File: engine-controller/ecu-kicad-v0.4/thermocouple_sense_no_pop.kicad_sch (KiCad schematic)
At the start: 5 parts, among them U1 AD8495

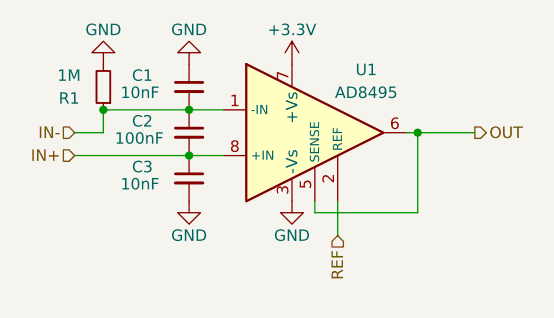
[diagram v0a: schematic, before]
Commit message: Progress on ECU v0.4
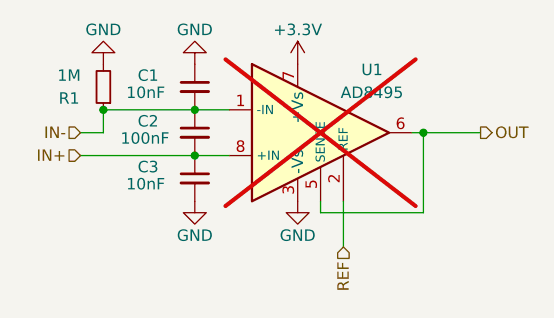
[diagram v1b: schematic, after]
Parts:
- U1: footprint Package_SO:MSOP-8_3x3mm_P0.65mm -> CustomFootprints:MSOP-8_3x3mm_P0.65mm_HandSolder; now not fitted
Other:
- moved on the sheet: C1, C2, C3
